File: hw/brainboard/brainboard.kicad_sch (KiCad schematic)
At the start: 6 parts, among them J3 gpio, J4 misc, J5 inputs, J6 audio_dac_power, J7 eurorack_power

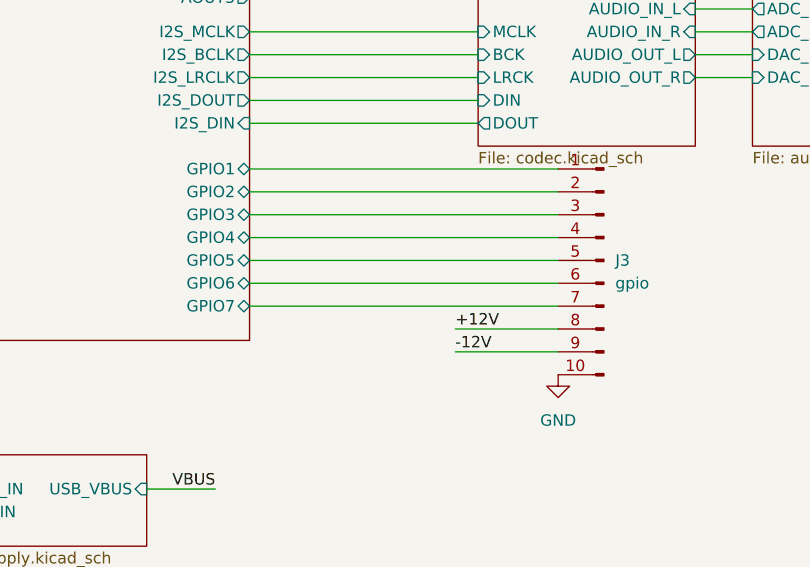
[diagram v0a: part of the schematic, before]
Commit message: Brainboard polishing
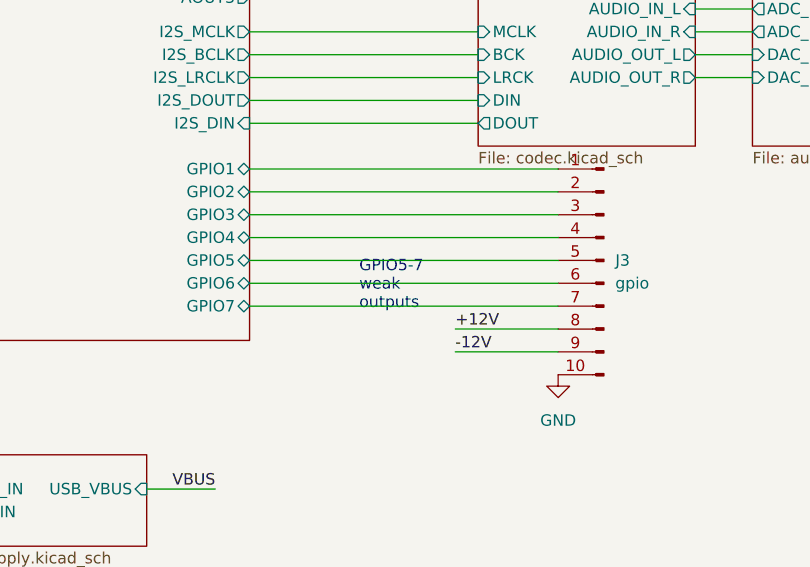
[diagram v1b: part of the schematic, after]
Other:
- note added: "GPIO5-7 weak outputs"
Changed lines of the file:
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@@
 		(company "Jonas Norling")
+	)
+	(text "GPIO5-7\nweak\noutputs"
+		(exclude_from_sim no)
+		(at 146.812 124.714 0)
+		(effects
+			(font
+				(size 1.27 1.27)
+			)
+			(justify left)
+		)
 	)
 	(wire
